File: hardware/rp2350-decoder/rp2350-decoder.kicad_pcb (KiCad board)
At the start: 6 copper layers, 19.9 x 8.8 mm, 67 parts, among them J1 SWDIO, J2 SWCLK, J3 5052702412, Q1 DMN2991UDA-7B, Q2 DMN2991UDA-7B, Q3 NST847BPDP6T5G, Q4 NST847BPDP6T5G, Q5 DMN2991UDA-7B, Q6 DMN2991UDA-7B, Q7 DMN2991UDA-7B, Q8 DMN2991UDA-7B, SW1 BOOT, U1 NCS2220AMUT1G, U2 AP63203WU, U3 W25Q128JVPIQ, U4 RP2350A, U5 MAX98357AEWL+T, U6 MD9927, Y1 X252012MMB4SI

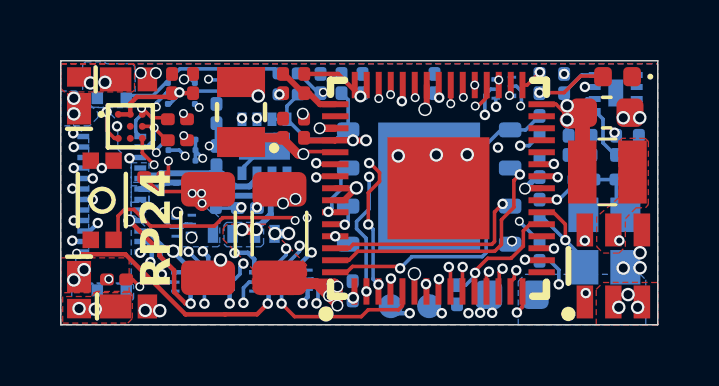
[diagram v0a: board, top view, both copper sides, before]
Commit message: chore: pcb cleanup
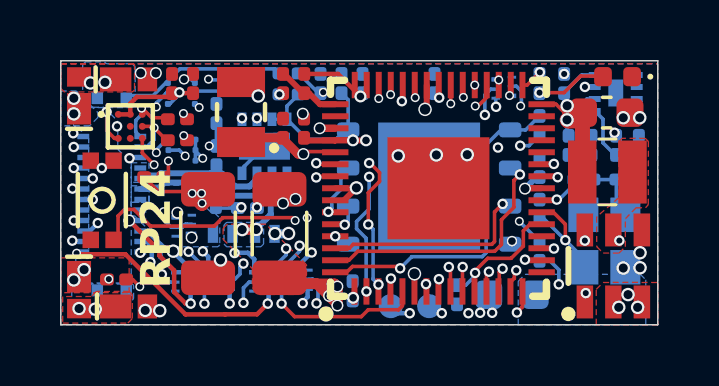
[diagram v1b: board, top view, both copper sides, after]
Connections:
- net /GPIO21 renamed /DCC_TTL
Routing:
- net GND: track 7.85 -> 6.09 mm
- net +3.3V: track 30.9 -> 29.6 mm
- net /CAP_VDC: track 11.8 -> 10.9 mm
- net /QSPI_CS: track 11.1 -> 10.4 mm
